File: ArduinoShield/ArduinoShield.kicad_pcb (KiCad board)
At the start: 2 copper layers, 100 x 60 mm, 3 parts, among them J1 Conn_02x15_Odd_Even, J2 Conn_01x04

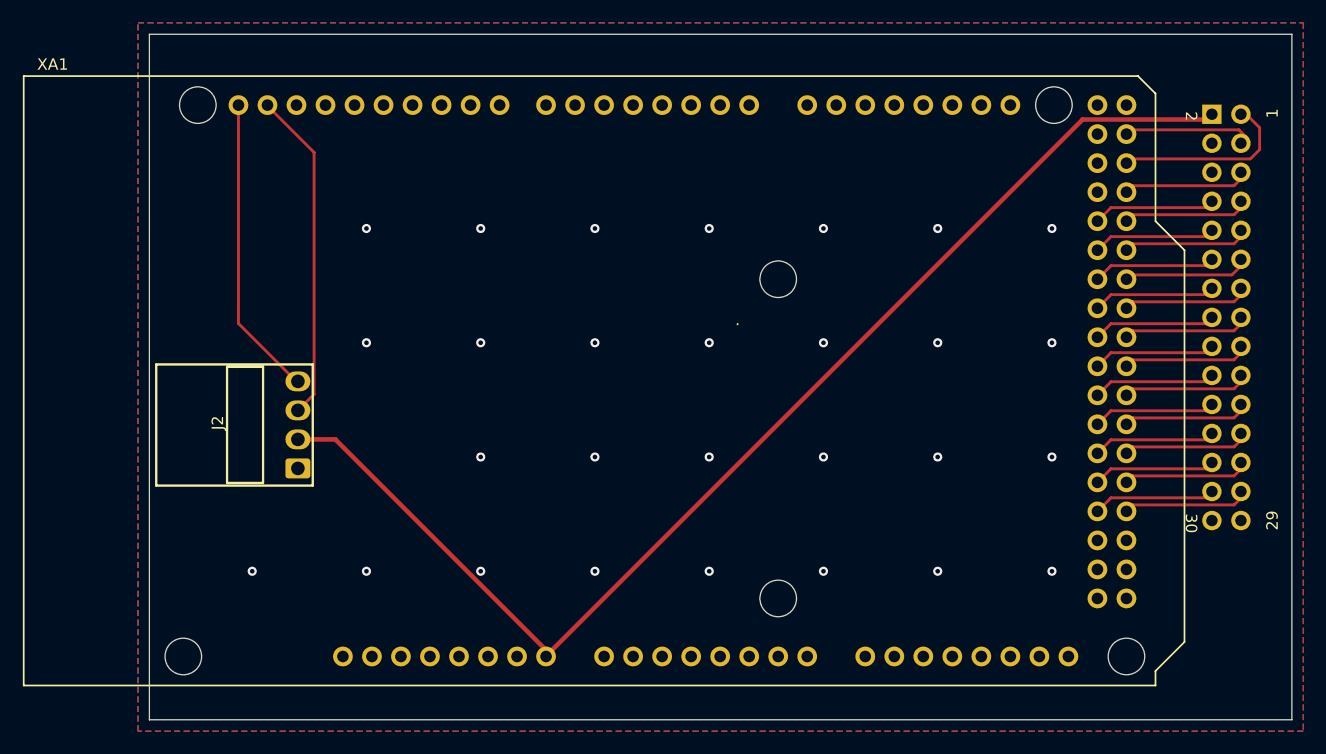
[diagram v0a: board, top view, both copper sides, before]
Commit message: Finally done maybe for real
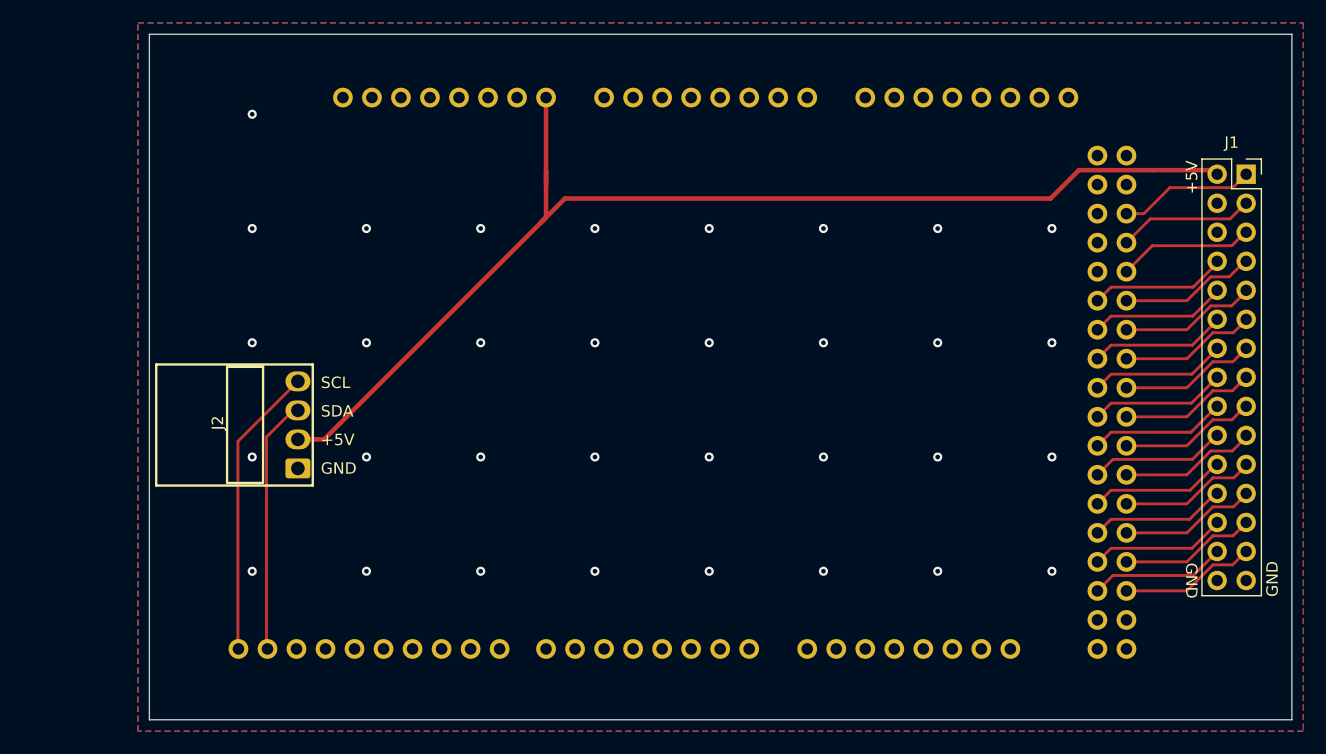
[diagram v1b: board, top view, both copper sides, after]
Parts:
- J1: moved to F.Cu
- XA1: moved to B.Cu
- moved XA1 54.0 mm to (100.0, 66.0)
- moved J1 6.05 mm to (207.0, 75.2), turned to 0 degrees
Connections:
- XA1 pad D23: CLK -> Net-(XA1-PadD23)
- XA1 pad D24: Net-(XA1-PadD24) -> IDENT2_SW
- XA1 pad D25: CS_LOAD -> IDENT1_SW
- XA1 pad D26: Net-(XA1-PadD26) -> RADIO2_LED
- XA1 pad D27: DIN -> RADIO1_LED
- XA1 pad D28: COMM2_LEFT -> RADIO2_SW
- XA1 pad D29: COMM1_LEFT -> RADIO1_SW
- XA1 pad D30: COMM2_RIGHT -> NAV2_XFR
- XA1 pad D31: COMM1_RIGHT -> NAV1_XFR
- XA1 pad D32: COMM2_KHZ_SW -> NAV2_KHZ_SW
- XA1 pad D33: COMM1_KHZ_SW -> NAV1_KHZ_SW
- XA1 pad D34: COMM2_XFR -> NAV2_RIGHT
- XA1 pad D35: COMM1_XFR -> NAV1_RIGHT
- XA1 pad D38: NAV2_RIGHT -> COMM2_XFR
- XA1 pad D39: NAV1_RIGHT -> COMM1_XFR
- XA1 pad D40: NAV2_KHZ_SW -> COMM2_KHZ_SW
- XA1 pad D41: NAV1_KHZ_SW -> COMM1_KHZ_SW
- XA1 pad D42: NAV2_XFR -> COMM2_RIGHT
- XA1 pad D43: NAV1_XFR -> COMM1_RIGHT
- XA1 pad D44: RADIO2_SW -> COMM2_LEFT
- XA1 pad D45: RADIO1_SW -> COMM1_LEFT
- XA1 pad D46: RADIO2_LED -> Net-(XA1-PadD46)
- XA1 pad D47: RADIO1_LED -> DIN
- XA1 pad D48: IDENT2_SW -> Net-(XA1-PadD48)
- XA1 pad D49: IDENT1_SW -> CLK
- XA1 pad D51: Net-(XA1-PadD51) -> CS_LOAD
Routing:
- net SDA: track 28.8 -> 22.2 mm
- net +5V: track 108.5 -> 102.7 mm
- net CS_LOAD: track 15.7 -> 11.9 mm
- net CLK: track 10.9 -> 11.9 mm
- net COMM2_RIGHT: track 10.9 -> 11.9 mm
- net SCL: track 26.7 -> 25.8 mm
- net RADIO2_SW: track 11.2 -> 12.0 mm
- net NAV2_XFR: track 11.2 -> 12.0 mm
- net NAV2_KHZ_SW: track 11.2 -> 12.0 mm
- net NAV2_RIGHT: track 11.2 -> 12.0 mm
- net COMM1_LEFT: track 11.2 -> 12.0 mm
- net DIN: track 11.2 -> 11.9 mm
- net COMM2_XFR: track 11.2 -> 11.9 mm
- net RADIO2_LED: track 11.2 -> 11.9 mm
- net NAV1_RIGHT: track 11.2 -> 11.9 mm
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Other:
- net class +5V added: clearance 0.2, trace_width 0.4, via_dia 0.8, via_drill 0.4
- net class GND added: clearance 0.2, trace_width 0.4, via_dia 0.8, via_drill 0.4
- board text added: "+5V"
- board text added: "GND"
- board text added: "SCL"
- board text added: "SDA"
- board text removed: "1"
- board text removed: "2"
- board text removed: "29"
- board text removed: "30"

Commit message: Final version submitted for assembly
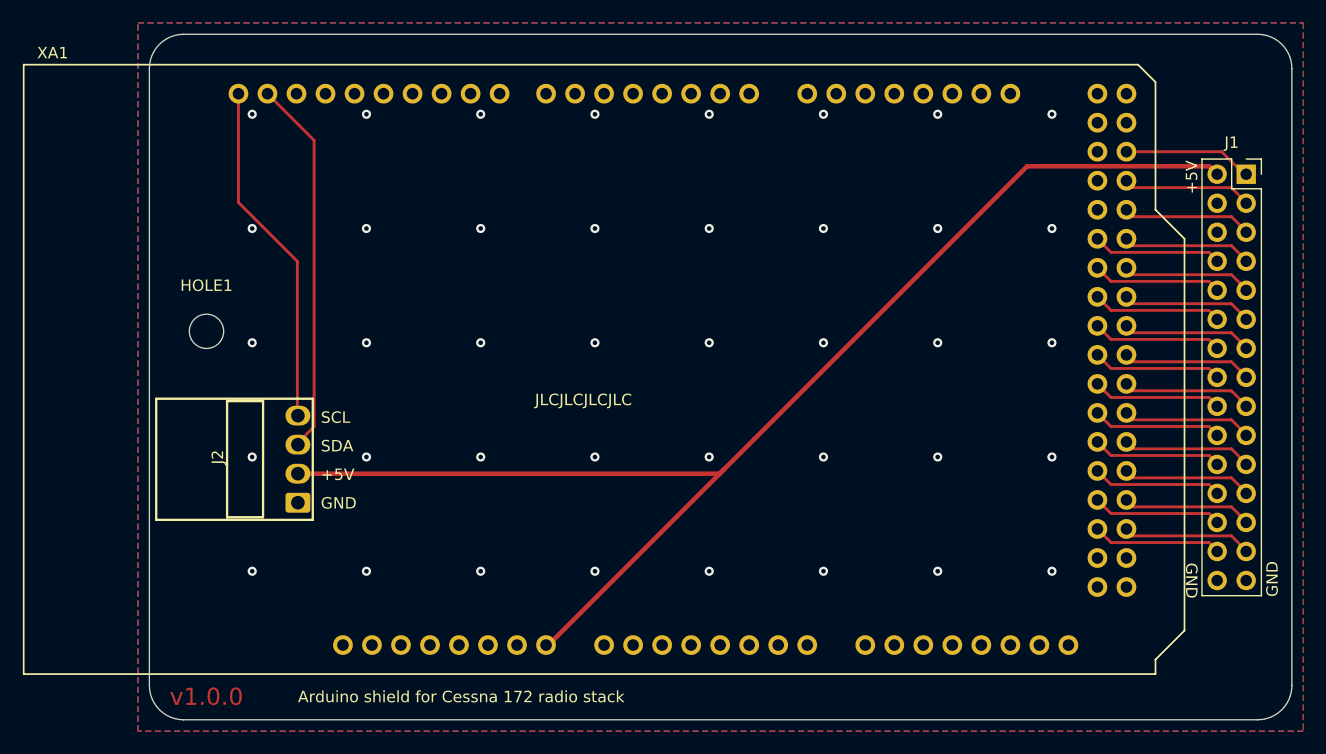
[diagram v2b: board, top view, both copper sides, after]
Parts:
- added HOLE1: MountingHole_3mm, MountingHole:MountingHole_3mm, F.Cu at (116.0, 89.0)
- XA1: moved to F.Cu
- moved XA1 53.0 mm to (100.0, 119.0)
- moved J2 3.00 mm to (124.0, 104.0)
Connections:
- XA1 pad D24: IDENT2_SW -> Net-(XA1-PadD24)
- XA1 pad D25: IDENT1_SW -> CS_LOAD
- XA1 pad D26: RADIO2_LED -> Net-(XA1-PadD26)
- XA1 pad D27: RADIO1_LED -> CLK
- XA1 pad D28: RADIO2_SW -> Net-(XA1-PadD28)
- XA1 pad D29: RADIO1_SW -> DIN
- XA1 pad D30: NAV2_XFR -> COMM2_LEFT
- XA1 pad D31: NAV1_XFR -> COMM1_LEFT
- XA1 pad D32: NAV2_KHZ_SW -> COMM2_RIGHT
- XA1 pad D33: NAV1_KHZ_SW -> COMM1_RIGHT
- XA1 pad D34: NAV2_RIGHT -> COMM2_KHZ_SW
- XA1 pad D35: NAV1_RIGHT -> COMM1_KHZ_SW
- XA1 pad D36: NAV2_LEFT -> COMM2_XFR
- XA1 pad D37: NAV1_LEFT -> COMM1_XFR
- XA1 pad D38: COMM2_XFR -> NAV2_LEFT
- XA1 pad D39: COMM1_XFR -> NAV1_LEFT
- XA1 pad D40: COMM2_KHZ_SW -> NAV2_RIGHT
- XA1 pad D41: COMM1_KHZ_SW -> NAV1_RIGHT
- XA1 pad D42: COMM2_RIGHT -> NAV2_KHZ_SW
- XA1 pad D43: COMM1_RIGHT -> NAV1_KHZ_SW
- XA1 pad D44: COMM2_LEFT -> NAV2_XFR
- XA1 pad D45: COMM1_LEFT -> NAV1_XFR
- XA1 pad D46: Net-(XA1-PadD46) -> RADIO2_SW
- XA1 pad D47: DIN -> RADIO1_SW
- XA1 pad D48: Net-(XA1-PadD48) -> RADIO2_LED
- XA1 pad D49: CLK -> RADIO1_LED
- XA1 pad D50: Net-(XA1-PadD50) -> IDENT2_SW
- XA1 pad D51: CS_LOAD -> IDENT1_SW
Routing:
- net +5V: track 102.7 -> 113.8 mm
- net SDA: track 22.2 -> 32.9 mm
- net SCL: track 25.8 -> 30.2 mm
- net RADIO2_SW: track 12.0 -> 11.3 mm
- net NAV2_XFR: track 12.0 -> 11.3 mm
- net NAV2_KHZ_SW: track 12.0 -> 11.3 mm
- net NAV2_RIGHT: track 12.0 -> 11.3 mm
- net NAV2_LEFT: track 12.0 -> 11.3 mm
- net COMM1_LEFT: track 12.0 -> 11.3 mm
- net IDENT2_SW: track 12.0 -> 11.3 mm
- net DIN: track 11.9 -> 11.3 mm
- net COMM2_XFR: track 11.9 -> 11.3 mm
- net RADIO2_LED: track 11.9 -> 11.3 mm
- net NAV1_RIGHT: track 11.9 -> 11.3 mm
- net COMM2_KHZ_SW: track 11.9 -> 11.3 mm
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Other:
- outline, holes or cut-outs redrawn
- board text added: "Arduino shield for Cessna 172 radio stack"
- board text added: "JLCJLCJLCJLC"
- board text added: "v1.0.0"
